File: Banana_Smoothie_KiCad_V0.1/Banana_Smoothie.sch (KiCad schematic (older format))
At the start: 120 parts, among them IC1 LPC1769, IC5 LD117ADT33TR, Q1 BSL207SP, Q2 12MHz, SW1 SW_TACT_4P_B, SW3 SW_TACT_4P_B, U3 USD-SOCKETUSD, X14 USB

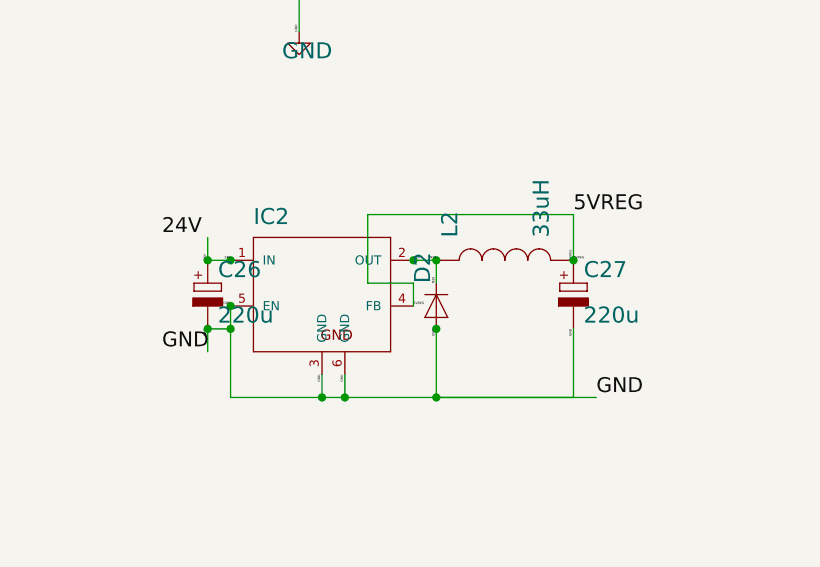
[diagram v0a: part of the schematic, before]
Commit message: Added LAN8720_Module
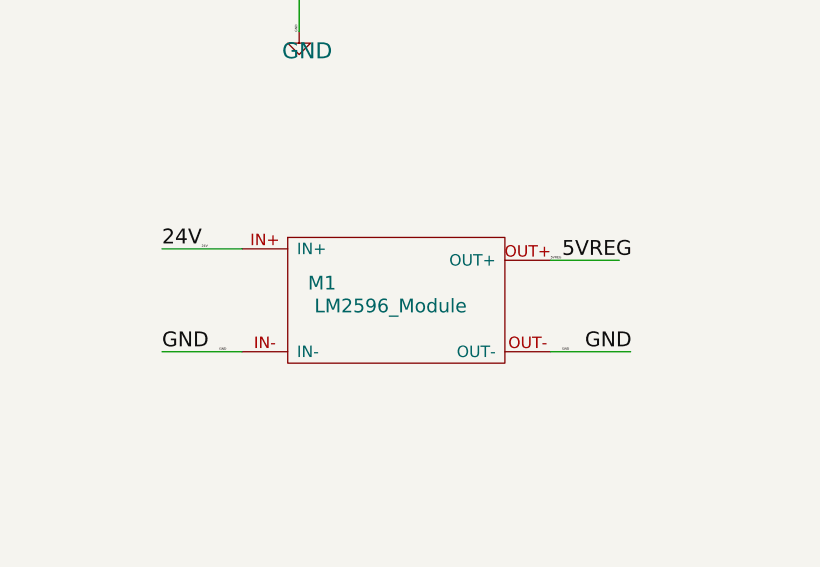
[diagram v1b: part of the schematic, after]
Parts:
- removed C26, C27: 220u, RCL_E2_5-7, symbol RCL_CPOL-EU
- removed D2: 214AC, DP_DEVICES_DO-214AC, symbol DP_DEVICES_DIODE
- removed IC2: ~, SmoothieBrainz - next round:LINEAR_TO263-5, symbol LINEAR_LM2596S
- removed L2: 33uH, SPARKFUN-PASSIVES_CDRH125, symbol SPARKFUN-PASSIVES_INDUCTOR
- added M1: LM2596_Module, Banana_Smoothie_Footprints:LM2596_Module, symbol LM2596_Module
- JP1: footprint PINHEAD_2X07_90 -> Banana_Smoothie_Footprints:LAN8720_Module
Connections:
- net labels removed: N$9
- wire segments 451 -> 437
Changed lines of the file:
@@
 EESchema Schematic File Version 2
-LIBS:Banana_SmoothieBrainz
+LIBS:Banana_Smoothie
 LIBS:power
 LIBS:Oscillators
@@
 $EndComp
 $Comp
-L RCL_CPOL-EU C26
-U 1 1 58522BC5
-P 19050 18150
-F 0 "C26" H 19095 18168 70  0000 L BNN
-F 1 "220u" H 19094 17969 70  0000 L BNN
-F 2 "RCL_E2_5-7" H 19040 17940 65  0001 L TNN
-F 3 "" H 19050 18150 60  0001 C CNN
-	1    19050 18150
-	1    0    0    -1
-$EndComp
-$Comp
-L RCL_CPOL-EU C27
-U 1 1 58522C8D
-P 20650 18150
-F 0 "C27" H 20695 18168 70  0000 L BNN
-F 1 "220u" H 20694 17969 70  0000 L BNN
-F 2 "RCL_E2_5-7" H 20640 17940 65  0001 L TNN
-F 3 "" H 20650 18150 60  0001 C CNN
-	1    20650 18150
-	1    0    0    -1
-$EndComp
-$Comp
 L RCL_C-EU C44
 U 1 1 58522E1D
@@
 $EndComp
 $Comp
-L DP_DEVICES_DIODE D2
-U 1 1 58523205
-P 20050 18250
-F 0 "D2" H 20150 18269 70  0000 L BNN
-F 1 "214AC" H 20040 18140 65  0001 L TNN
-F 2 "DP_DEVICES_DO-214AC" H 20040 18040 65  0001 L TNN
-F 3 "" H 20050 18250 60  0001 C CNN
-	1    20050 18250
-	0    -1   -1   0
-$EndComp
-$Comp
 L MICROBUILDER_DIODE D3
 U 1 1 585232CD
@@
 $EndComp
 $Comp
-L LINEAR_LM2596S IC2
-U 1 1 585241A5
-P 19550 18150
-F 0 "IC2" H 19250 18400 70  0000 L BNN
-F 1 "~" H 19540 18040 65  0001 L TNN
-F 2 "SmoothieBrainz - next round:LINEAR_TO263-5" H 19540 17940 65  0001 L TNN
-F 3 "" H 19550 18150 60  0001 C CNN
-	1    19550 18150
-	1    0    0    -1
-$EndComp
-$Comp
 L V-REG_LD117ADT33TR IC5
 U 1 1 5852426D
@@
 F 0 "JP1" H 12800 13574 70  0000 L BNN
 F 1 "JP1" H 13040 13040 65  0001 L TNN
-F 2 "PINHEAD_2X07_90" H 13040 12940 65  0001 L TNN
+F 2 "Banana_Smoothie_Footprints:LAN8720_Module" H 13040 12940 65  0001 L TNN
 F 3 "" H 13050 13150 60  0001 C CNN
 	1    13050 13150
@@
 $EndComp
 $Comp
-L SPARKFUN-PASSIVES_INDUCTOR L2
-U 1 1 5852507D
-P 20350 18050
-F 0 "L2" H 20450 18250 70  0000 L BNN
-F 1 "33uH" H 20450 17850 70  0000 L BNN
-F 2 "SPARKFUN-PASSIVES_CDRH125" H 20340 17840 65  0001 L TNN
-F 3 "" H 20350 18050 60  0001 C CNN
-	1    20350 18050
-	0    -1   -1   0
-$EndComp
-$Comp
 L LED_LED LED1
 U 1 1 58525145
@@
 Text Label 19050 16270 2    94   ~ 0
 5V
-Wire Wire Line
-	19950 18250 19950 18150
-Wire Wire Line
-	19950 18150 19750 18150
-Wire Wire Line
-	19750 18150 19750 17850
-Wire Wire Line
-	19750 17850 20650 17850
-Wire Wire Line
-	20650 17850 20650 18050
-Connection ~ 20650 18050
-Text Label 20650 17850 0    65   ~ 0
+Text Label 20600 18050 0    65   ~ 0
 5VREG
 Wire Wire Line
@@
 Text Label 11750 12950 0    65   ~ 0
 24V
-Wire Wire Line
-	19150 18050 19050 18050
-Wire Wire Line
-	19050 18050 19050 17950
-Connection ~ 19150 18050
-Connection ~ 19050 18050
-Text Label 18850 17950 0    65   ~ 0
+Text Label 18850 18000 0    65   ~ 0
 24V
 Wire Wire Line
@@
 GND
 Wire Wire Line
-	19150 18250 19150 18650
-Wire Wire Line
-	19150 18650 20650 18650
-Wire Wire Line
-	19550 18650 19550 18550
-Wire Wire Line
-	19650 18650 19650 18550
-Wire Wire Line
-	20050 18650 20050 18350
-Wire Wire Line
-	19150 18350 19050 18350
-Wire Wire Line
-	19050 18350 19050 18450
-Wire Wire Line
-	20050 18650 20750 18650
-Wire Wire Line
-	20650 18650 20650 18350
-Connection ~ 19550 18650
-Connection ~ 19650 18650
-Connection ~ 19150 18350
-Connection ~ 19150 18250
-Connection ~ 20050 18350
-Connection ~ 20050 18650
-Connection ~ 19050 18350
+	20900 18450 20550 18450
 Text Label 18850 18450 0    65   ~ 0
 GND
-Text Label 20750 18650 0    65   ~ 0
+Text Label 20700 18450 0    65   ~ 0
 GND
 Wire Wire Line
@@
 	16150 14950 16150 14750
 Wire Wire Line
-	19950 18050 20050 18050
-Wire Wire Line
-	20050 18050 20050 18150
-Connection ~ 20050 18050
-Connection ~ 19950 18050
-Wire Wire Line
 	16350 14950 16350 14750
 Wire Wire Line
@@
 Text GLabel 18750 16250 2    10   UnSpc ~ 0
 5V
-Text Label 20650 18050 0    10   ~ 0
-5VREG
-Text Label 19950 18250 0    10   ~ 0
-5VREG
-Text Label 20650 18050 1    10   ~ 0
+Text Label 20550 18050 0    10   ~ 0
 5VREG
 Text Label 18550 16250 2    10   ~ 0
@@
 Text Label 10950 12950 0    10   ~ 0
 24V
-Text Label 19150 18050 2    10   ~ 0
-24V
-Text Label 19050 18050 1    10   ~ 0
+Text Label 19050 18000 2    10   ~ 0
 24V
 Text Label 24950 23700 0    10   ~ 0
@@
 Text Label 10950 12550 0    10   ~ 0
 GND
-Text Label 19150 18250 2    10   ~ 0
-GND
-Text Label 19550 18550 3    10   ~ 0
-GND
-Text Label 19650 18550 3    10   ~ 0
+Text Label 19100 18450 0    10   ~ 0
 GND
-Text Label 20050 18350 3    10   ~ 0
-GND
-Text Label 19050 18350 3    10   ~ 0
-GND
-Text Label 20650 18350 3    10   ~ 0
+Text Label 20600 18450 0    10   ~ 0
 GND
 Text Label 10550 16950 1    10   ~ 0
@@
 Text Label 16150 14750 3    10   ~ 0
 N$8
-Text Label 19950 18050 0    10   ~ 0
-N$9
-Text Label 20050 18150 1    10   ~ 0
-N$9
-Text Label 20050 18050 2    10   ~ 0
-N$9
 Text Label 16350 14950 1    10   ~ 0
 N$10
@@
 	1    0    0    -1
 $EndComp
+$Comp
+L LM2596_Module M1
+U 1 1 5880D194
+P 19850 18250
+F 0 "M1" H 19550 18350 60  0000 C CNN
+F 1 "LM2596_Module" H 19850 18250 60  0000 C CNN
+F 2 "Banana_Smoothie_Footprints:LM2596_Module" H 19850 18250 60  0001 C CNN
+F 3 "" H 19850 18250 60  0001 C CNN
+	1    19850 18250
+	1    0    0    -1
+$EndComp
+Wire Wire Line
+	20550 18050 20850 18050
+Wire Wire Line
+	19200 18000 18850 18000
+Wire Wire Line
+	19200 18450 18850 18450
 $EndSCHEMATC
